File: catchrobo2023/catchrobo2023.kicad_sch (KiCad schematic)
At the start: 19 parts

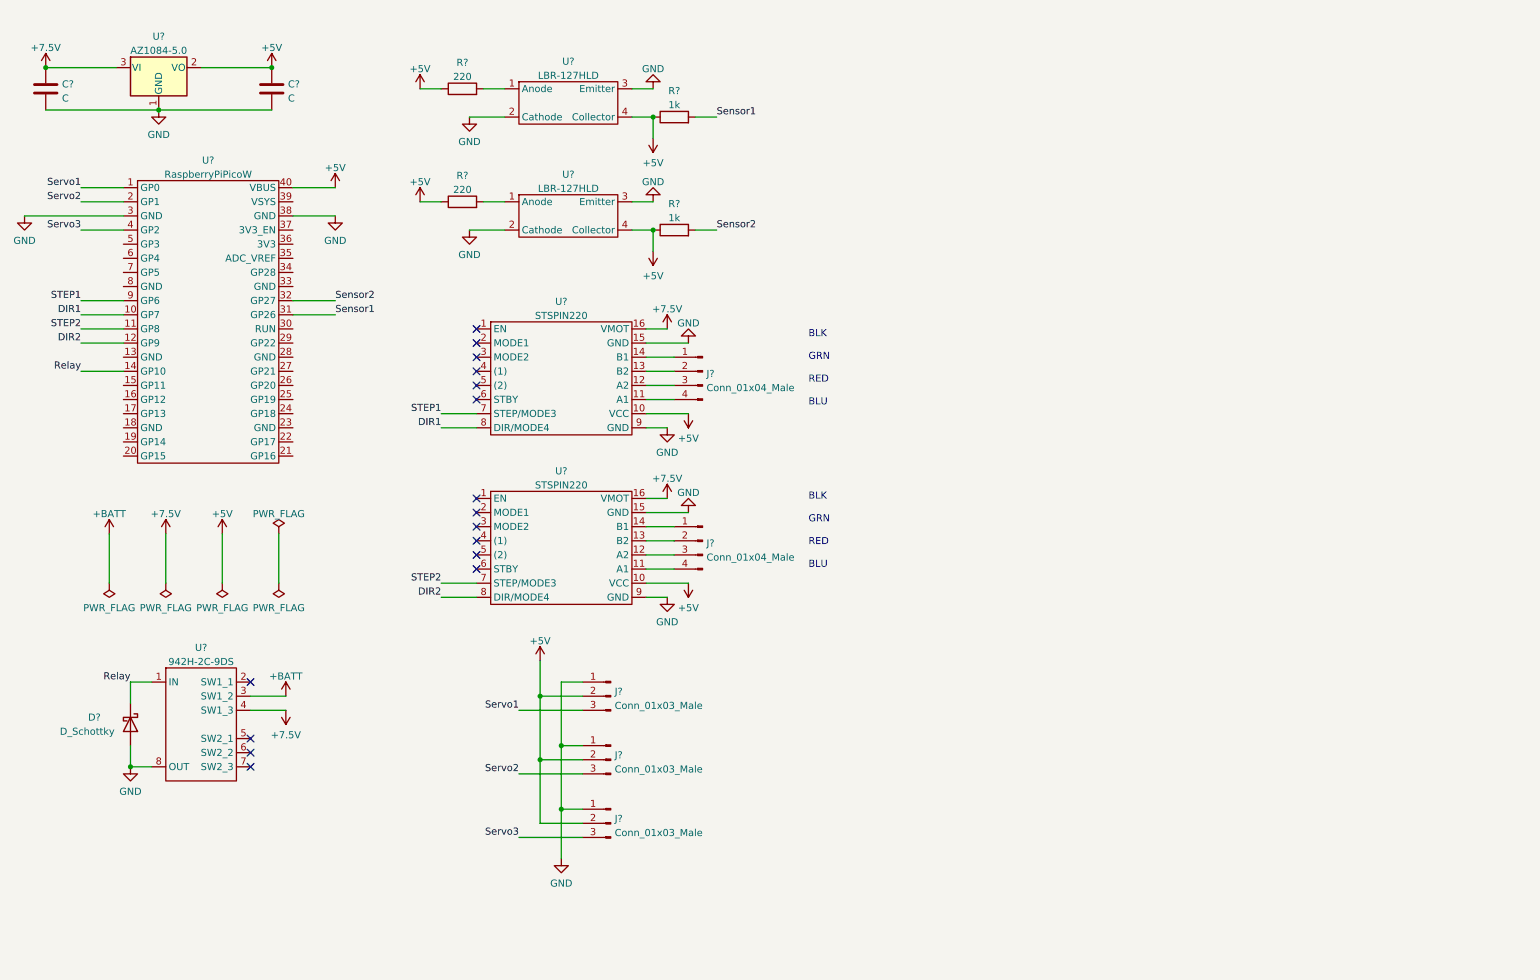
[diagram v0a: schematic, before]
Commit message: 緊急非常停止以外の回路図は完了
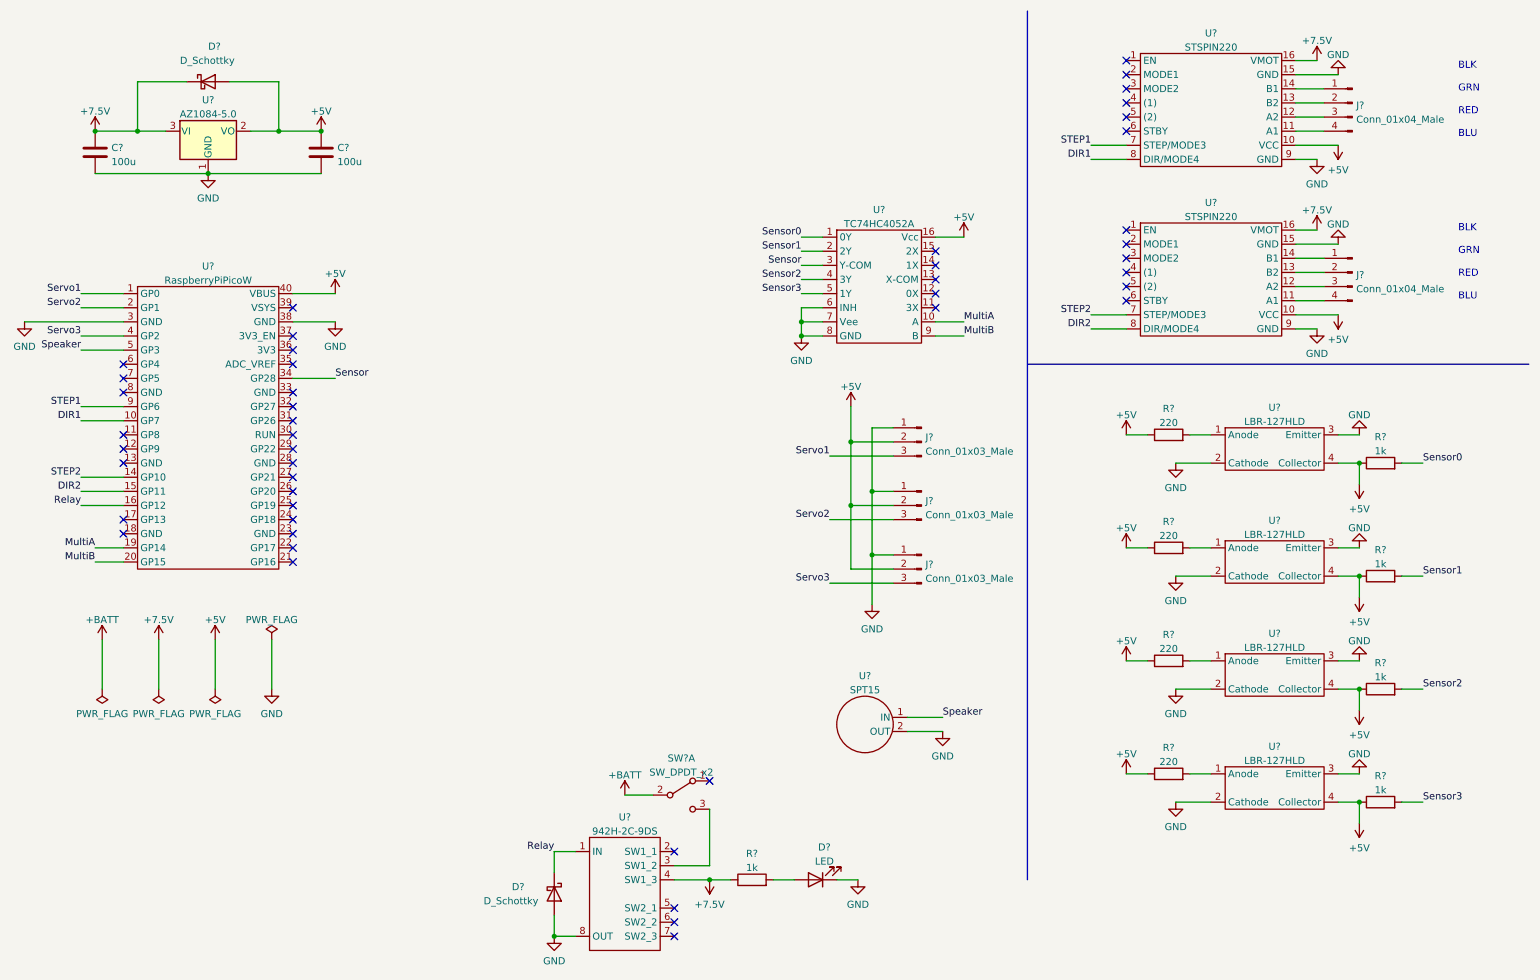
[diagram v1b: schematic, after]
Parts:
- added D?: LED, symbol Device:LED
- added D?: D_Schottky, symbol Device:D_Schottky
- added R? (x2): 220, symbol Device:R
- added R? (x3): 1k, symbol Device:R
- added SW?: SW_DPDT_x2, symbol Switch:SW_DPDT_x2
- added U?: SPT15, symbol catchrobo_parts:SPT15
- added U? (x2): LBR-127HLD, symbol catchrobo_parts:LBR-127HLD
- added U?: TC74HC4052A, symbol catchrobo_parts:TC74HC4052A
- C? (x2): value C -> 100u
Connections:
- net +5V: now also D?.2 (A), R?.1, R?.1, R?.1, R?.1, U?.16 (Vcc), U?.4 (Collector), U?.4 (Collector)
- net +7.5V: now also D?.1 (K), R?.1
- net +BATT: now also SW?.2 (B); no longer U?.3 (SW1_2)
- net DIR2: now also U?.15 (GP11); no longer U?.12 (GP9)
- net GND: now also D?.1 (K), U?.2 (Cathode), U?.2 (Cathode), U?.2 (OUT), U?.3 (Emitter), U?.3 (Emitter), U?.6 (INH), U?.7 (Vee), U?.8 (GND)
- net Relay: now also U?.16 (GP12); no longer U?.14 (GP10)
- net STEP2: now also U?.14 (GP10); no longer U?.11 (GP8)
- net Sensor1: now also U?.2 (2Y); no longer U?.31 (GP26)
- net Sensor2: now also U?.4 (3Y); no longer U?.32 (GP27)
- net MultiA: now reaches U?.19 (GP14)
- net MultiA: now also U?.10 (A)
- net MultiB: now reaches U?.20 (GP15)
- net MultiB: now also U?.9 (B)
- net Sensor: now reaches U?.34 (GP28)
- net Sensor: now also U?.3 (Y-COM)
- net Speaker: now reaches U?.5 (GP3)
- net Speaker: now also U?.1 (IN)
- new net: R?.2, U?.1 (Anode) (x2)
- new net: SW?.3 (C), U?.3 (SW1_2)
- new net: D?.2 (A), R?.2
- new net Sensor0: R?.2, U?.1 (0Y)
- new net Sensor3: R?.2, U?.5 (1Y)
- no-connect marks 16 -> 47
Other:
- moved on the sheet: C?, D?, J?, R?, U?
